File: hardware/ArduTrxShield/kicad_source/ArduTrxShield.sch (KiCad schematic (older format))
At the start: 74 parts, among them CN1 60312202114509, CN2 ARDUINO, CN3 CON_KLINKE3, CN4 CON_KLINKE3, CN5 CONN_01X03, CN6 CONN_01X02, IC1 SN74LVC1T45, IC2 SN74LVC1T45, Q1 2N7002, Q2 2N7002, Q3 2N7002, SW1 TAST_HOR, SW2 ALPS_EC11E, U1 DRA818, U2 LT1085, U3 LM4871

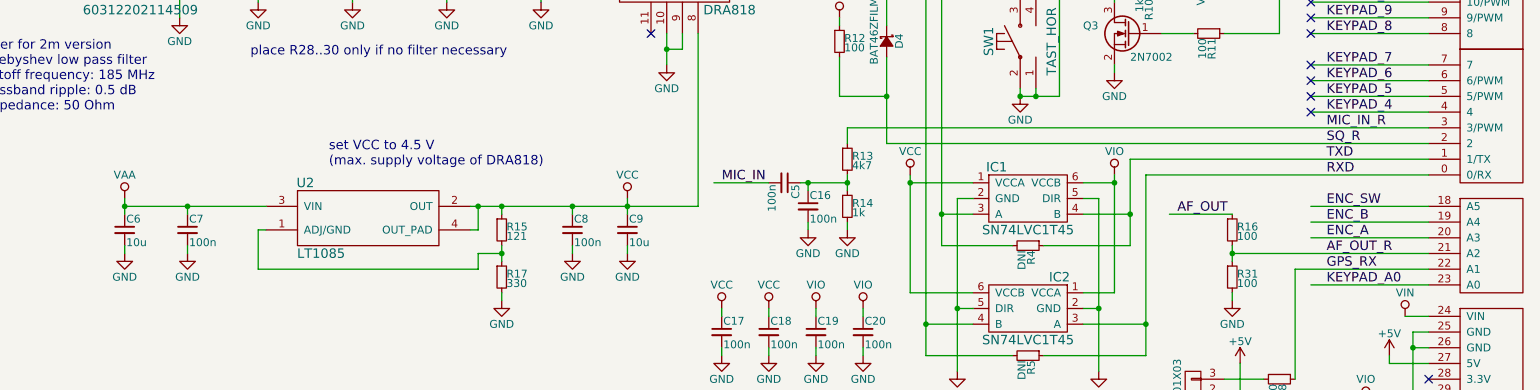
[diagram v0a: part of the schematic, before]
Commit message: updated layout and schematic
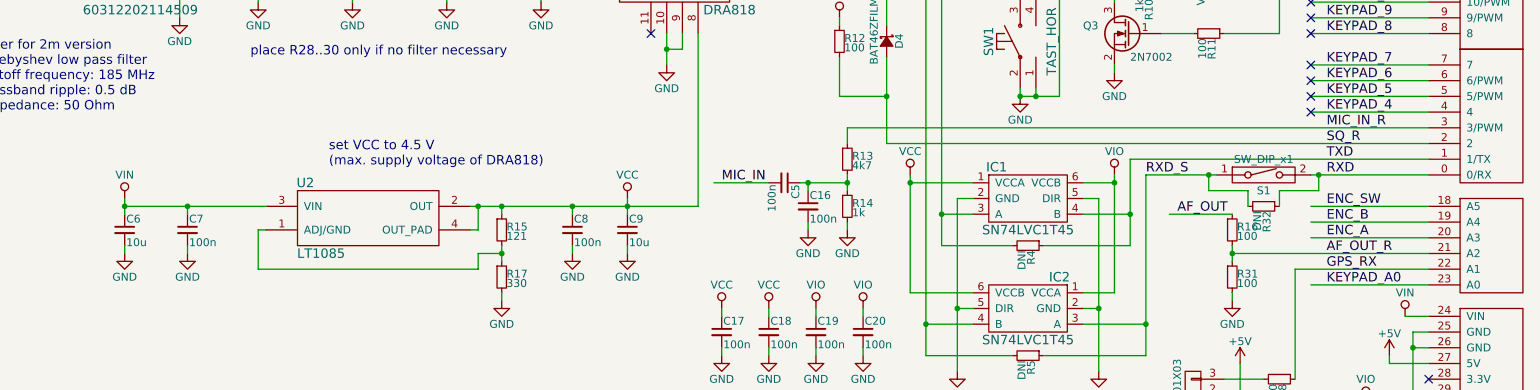
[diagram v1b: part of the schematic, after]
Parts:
- added R32: DNI, resistors:R_0603, symbol R_1206
- added S1: SW_DIP_x1, mechanical-switches:dip_1-300, symbol SW_DIP_x1
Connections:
- net labels added: RXD_S
- net labels removed: VAA
- wire segments 237 -> 244
